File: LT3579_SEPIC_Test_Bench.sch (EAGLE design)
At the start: 160 parts

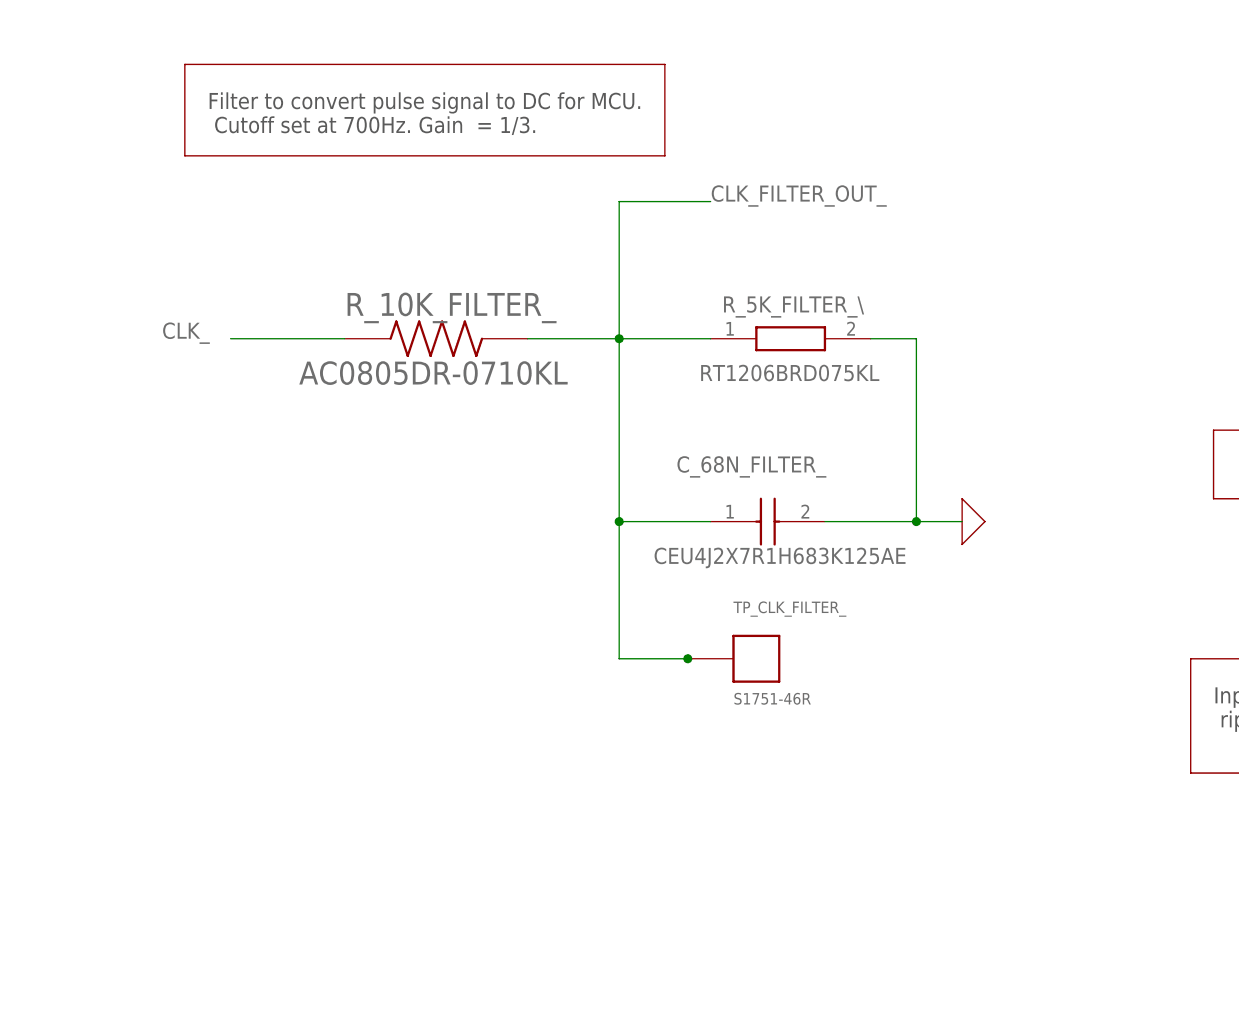
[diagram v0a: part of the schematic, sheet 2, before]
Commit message: modified routing
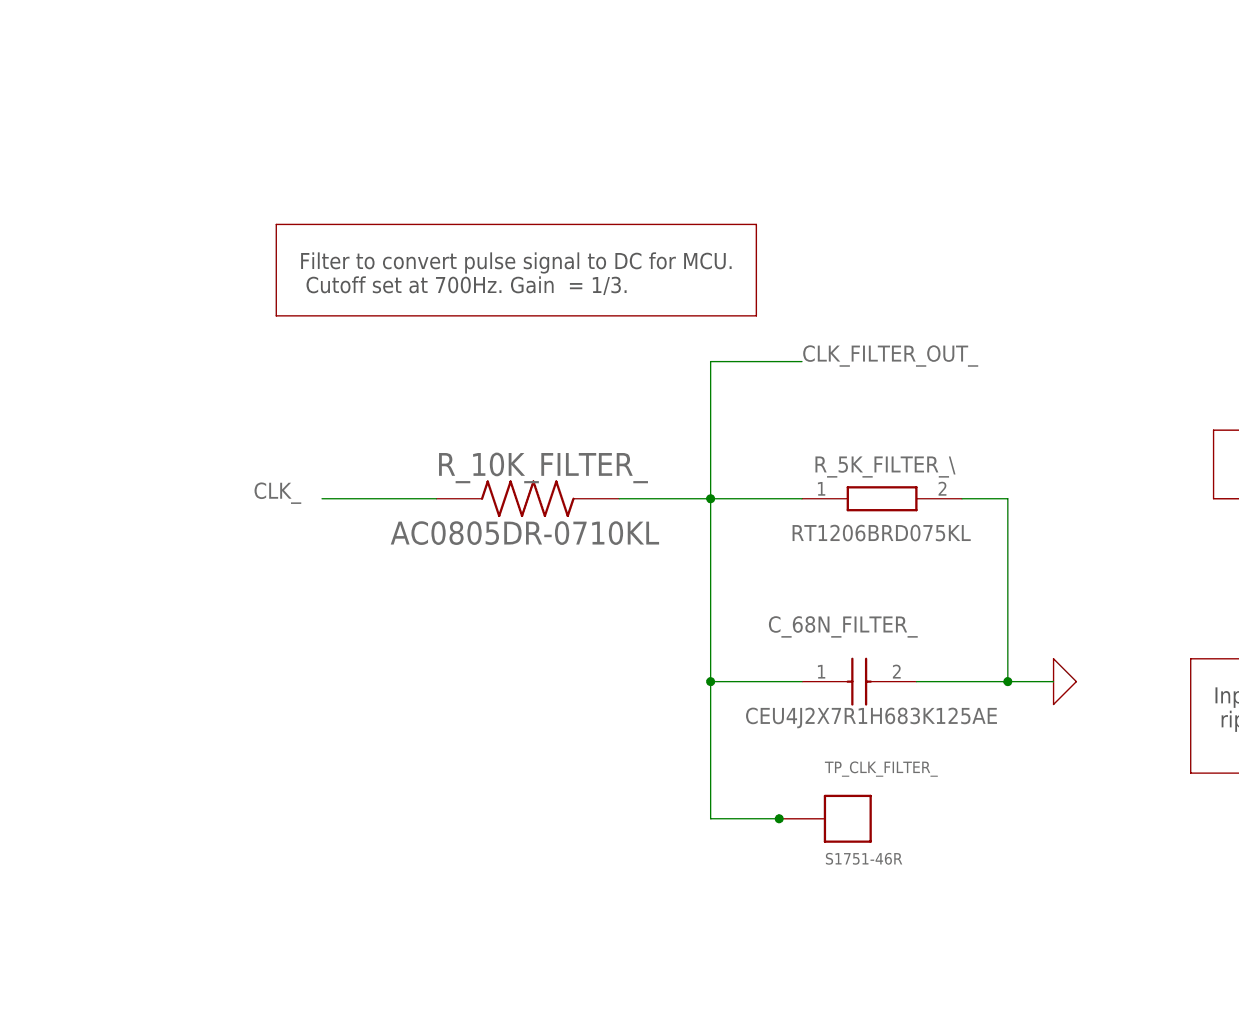
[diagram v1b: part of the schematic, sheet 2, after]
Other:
- moved on the sheet: C_68N_FILTER_, R_10K_FILTER_, R_5K_FILTER_\, TP_CLK_FILTER_
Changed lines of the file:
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@@
 <text x="-22.86" y="25.4" size="1.778" layer="95">LT3579 SEPIC Config: 13Vin -&gt; 14Vout</text>
 <text x="152.4" y="-5.08" size="1.778" layer="97">Ground Test Points</text>
-<text x="-208.28" y="147.32" size="1.778" layer="97">Filter to convert pulse signal to DC for MCU.
+<text x="-198.12" y="129.54" size="1.778" layer="97">Filter to convert pulse signal to DC for MCU.
  Cutoff set at 700Hz. Gain  = 1/3.</text>
 <text x="-205.74" y="-53.34" size="1.778" layer="97">13V -&gt; 3.3V output</text>
 <text x="-152.4" y="27.94" size="1.778" layer="97">Logic Level Shifter. 13V to 3.3V for MCU.</text>
 <text x="154.94" y="121.92" size="1.778" layer="97">20K + 5.6K Series Resistance</text>
-<wire x1="-210.82" y1="154.94" x2="-210.82" y2="144.78" width="0.1524" layer="94"/>
-<wire x1="-210.82" y1="144.78" x2="-157.48" y2="144.78" width="0.1524" layer="94"/>
-<wire x1="-157.48" y1="144.78" x2="-157.48" y2="154.94" width="0.1524" layer="94"/>
-<wire x1="-157.48" y1="154.94" x2="-210.82" y2="154.94" width="0.1524" layer="94"/>
+<wire x1="-200.66" y1="137.16" x2="-200.66" y2="127" width="0.1524" layer="94"/>
+<wire x1="-200.66" y1="127" x2="-147.32" y2="127" width="0.1524" layer="94"/>
+<wire x1="-147.32" y1="127" x2="-147.32" y2="137.16" width="0.1524" layer="94"/>
+<wire x1="-147.32" y1="137.16" x2="-200.66" y2="137.16" width="0.1524" layer="94"/>
 <wire x1="-154.94" y1="33.02" x2="-154.94" y2="25.4" width="0.1524" layer="94"/>
 <wire x1="-154.94" y1="25.4" x2="-104.14" y2="25.4" width="0.1524" layer="94"/>
@@
 <attribute name="VALUE" x="-10.16" y="147.32" size="1.27" layer="96"/>
 </instance>
-<instance part="R_10K_FILTER_" gate="G$1" x="-182.88" y="124.46" smashed="yes">
-<attribute name="NAME" x="-193.044440625" y="127.00148125" size="2.54148125" layer="95"/>
-<attribute name="VALUE" x="-198.12996875" y="119.373359375" size="2.54331875" layer="96"/>
-</instance>
-<instance part="R_5K_FILTER_\" gate="G$1" x="-152.4" y="124.46" smashed="yes">
-<attribute name="NAME" x="-151.13" y="128.27" size="1.778" layer="95" align="center-left"/>
-<attribute name="VALUE" x="-153.67" y="120.65" size="1.778" layer="96" align="center-left"/>
-</instance>
-<instance part="C_68N_FILTER_" gate="G$1" x="-152.4" y="104.14" smashed="yes">
-<attribute name="NAME" x="-156.21" y="110.49" size="1.778" layer="95" align="center-left"/>
-<attribute name="VALUE" x="-158.75" y="100.33" size="1.778" layer="96" align="center-left"/>
-</instance>
-<instance part="X_65" gate="G$1" x="-124.46" y="104.14" smashed="yes" rot="R90"/>
-<instance part="TP_CLK_FILTER_" gate="G$1" x="-147.32" y="88.9" smashed="yes">
-<attribute name="NAME" x="-149.86" y="93.98" size="1.27" layer="95"/>
-<attribute name="VALUE" x="-149.86" y="83.82" size="1.27" layer="96"/>
+<instance part="R_10K_FILTER_" gate="G$1" x="-172.72" y="106.68" smashed="yes">
+<attribute name="NAME" x="-182.884440625" y="109.22148125" size="2.54148125" layer="95"/>
+<attribute name="VALUE" x="-187.96996875" y="101.593359375" size="2.54331875" layer="96"/>
+</instance>
+<instance part="R_5K_FILTER_\" gate="G$1" x="-142.24" y="106.68" smashed="yes">
+<attribute name="NAME" x="-140.97" y="110.49" size="1.778" layer="95" align="center-left"/>
+<attribute name="VALUE" x="-143.51" y="102.87" size="1.778" layer="96" align="center-left"/>
+</instance>
+<instance part="C_68N_FILTER_" gate="G$1" x="-142.24" y="86.36" smashed="yes">
+<attribute name="NAME" x="-146.05" y="92.71" size="1.778" layer="95" align="center-left"/>
+<attribute name="VALUE" x="-148.59" y="82.55" size="1.778" layer="96" align="center-left"/>
+</instance>
+<instance part="X_65" gate="G$1" x="-114.3" y="86.36" smashed="yes" rot="R90"/>
+<instance part="TP_CLK_FILTER_" gate="G$1" x="-137.16" y="71.12" smashed="yes">
+<attribute name="NAME" x="-139.7" y="76.2" size="1.27" layer="95"/>
+<attribute name="VALUE" x="-139.7" y="66.04" size="1.27" layer="96"/>
 </instance>
 <instance part="R_LS_GATE_" gate="G$1" x="-175.26" y="15.24" smashed="yes">
@@
 <segment>
 <pinref part="C_68N_FILTER_" gate="G$1" pin="2"/>
-<wire x1="-139.7" y1="104.14" x2="-129.54" y2="104.14" width="0.1524" layer="91"/>
+<wire x1="-129.54" y1="86.36" x2="-119.38" y2="86.36" width="0.1524" layer="91"/>
 <pinref part="X_65" gate="G$1" pin="0"/>
 <pinref part="R_5K_FILTER_\" gate="G$1" pin="2"/>
-<wire x1="-129.54" y1="104.14" x2="-124.46" y2="104.14" width="0.1524" layer="91"/>
-<wire x1="-134.62" y1="124.46" x2="-129.54" y2="124.46" width="0.1524" layer="91"/>
-<wire x1="-129.54" y1="124.46" x2="-129.54" y2="104.14" width="0.1524" layer="91"/>
-<junction x="-129.54" y="104.14"/>
+<wire x1="-119.38" y1="86.36" x2="-114.3" y2="86.36" width="0.1524" layer="91"/>
+<wire x1="-124.46" y1="106.68" x2="-119.38" y2="106.68" width="0.1524" layer="91"/>
+<wire x1="-119.38" y1="106.68" x2="-119.38" y2="86.36" width="0.1524" layer="91"/>
+<junction x="-119.38" y="86.36"/>
 </segment>
 <segment>
@@
 <segment>
 <pinref part="R_10K_FILTER_" gate="G$1" pin="1"/>
-<wire x1="-193.04" y1="124.46" x2="-205.74" y2="124.46" width="0.1524" layer="91"/>
-<label x="-213.36" y="124.46" size="1.778" layer="95"/>
+<wire x1="-182.88" y1="106.68" x2="-195.58" y2="106.68" width="0.1524" layer="91"/>
+<label x="-203.2" y="106.68" size="1.778" layer="95"/>
 </segment>
 </net>
@@
 <pinref part="R_10K_FILTER_" gate="G$1" pin="2"/>
 <pinref part="R_5K_FILTER_\" gate="G$1" pin="1"/>
-<wire x1="-172.72" y1="124.46" x2="-162.56" y2="124.46" width="0.1524" layer="91"/>
+<wire x1="-162.56" y1="106.68" x2="-152.4" y2="106.68" width="0.1524" layer="91"/>
 <pinref part="C_68N_FILTER_" gate="G$1" pin="1"/>
-<wire x1="-162.56" y1="124.46" x2="-152.4" y2="124.46" width="0.1524" layer="91"/>
-<wire x1="-152.4" y1="104.14" x2="-162.56" y2="104.14" width="0.1524" layer="91"/>
-<wire x1="-162.56" y1="104.14" x2="-162.56" y2="124.46" width="0.1524" layer="91"/>
-<wire x1="-162.56" y1="124.46" x2="-162.56" y2="139.7" width="0.1524" layer="91"/>
-<wire x1="-162.56" y1="139.7" x2="-152.4" y2="139.7" width="0.1524" layer="91"/>
-<label x="-152.4" y="139.7" size="1.778" layer="95"/>
-<wire x1="-162.56" y1="104.14" x2="-162.56" y2="88.9" width="0.1524" layer="91"/>
+<wire x1="-152.4" y1="106.68" x2="-142.24" y2="106.68" width="0.1524" layer="91"/>
+<wire x1="-142.24" y1="86.36" x2="-152.4" y2="86.36" width="0.1524" layer="91"/>
+<wire x1="-152.4" y1="86.36" x2="-152.4" y2="106.68" width="0.1524" layer="91"/>
+<wire x1="-152.4" y1="106.68" x2="-152.4" y2="121.92" width="0.1524" layer="91"/>
+<wire x1="-152.4" y1="121.92" x2="-142.24" y2="121.92" width="0.1524" layer="91"/>
+<label x="-142.24" y="121.92" size="1.778" layer="95"/>
+<wire x1="-152.4" y1="86.36" x2="-152.4" y2="71.12" width="0.1524" layer="91"/>
 <pinref part="TP_CLK_FILTER_" gate="G$1" pin="1"/>
-<wire x1="-162.56" y1="88.9" x2="-154.94" y2="88.9" width="0.1524" layer="91"/>
-<junction x="-162.56" y="104.14"/>
-<junction x="-154.94" y="88.9"/>
-<junction x="-162.56" y="124.46"/>
-</segment>
-</net>
+<wire x1="-152.4" y1="71.12" x2="-144.78" y2="71.12" width="0.1524" layer="91"/>
+<junction x="-152.4" y="86.36"/>
+<junction x="-144.78" y="71.12"/>
+<junction x="-152.4" y="106.68"/>
+</segment>
+</net>
